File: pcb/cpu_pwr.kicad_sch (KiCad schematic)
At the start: 49 parts, among them J3 BATT, J4 Conn_01x02, J5 Conn_01x02, U7 AXP209

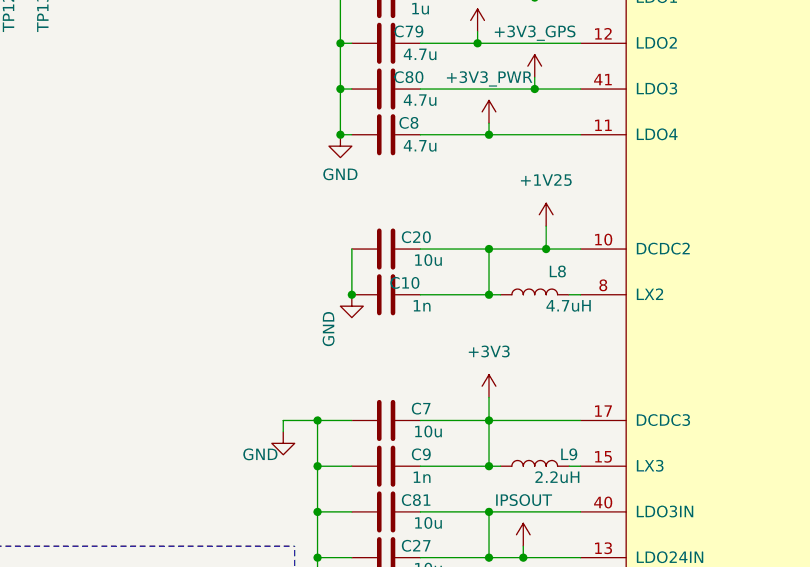
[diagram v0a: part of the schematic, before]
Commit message: Final fixes
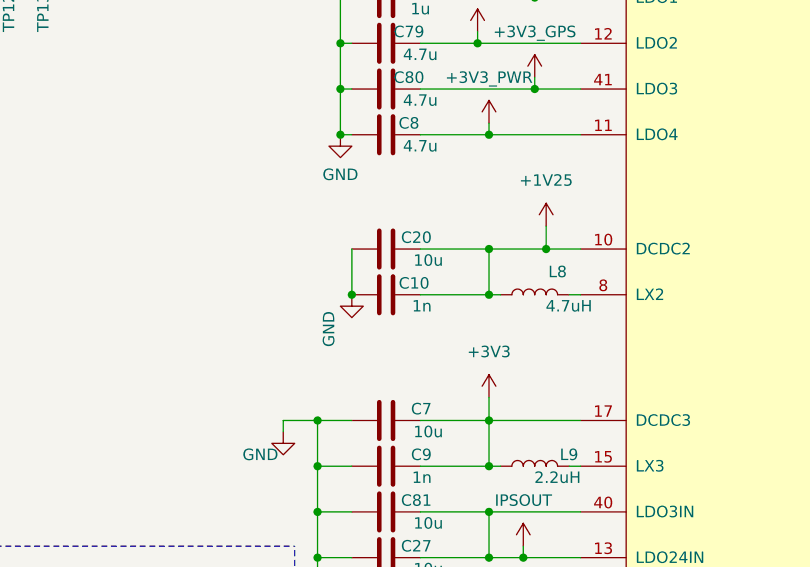
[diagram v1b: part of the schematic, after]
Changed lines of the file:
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@@
 		(dnp no)
 		(property "Reference" "C10"
-			(at 90.17 76.2 90)
+			(at 91.186 76.2 90)
 			(show_name no)
 			(do_not_autoplace no)
